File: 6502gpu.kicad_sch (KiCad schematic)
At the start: 1 part, among them J1 DE15_Receptacle_HighDensity

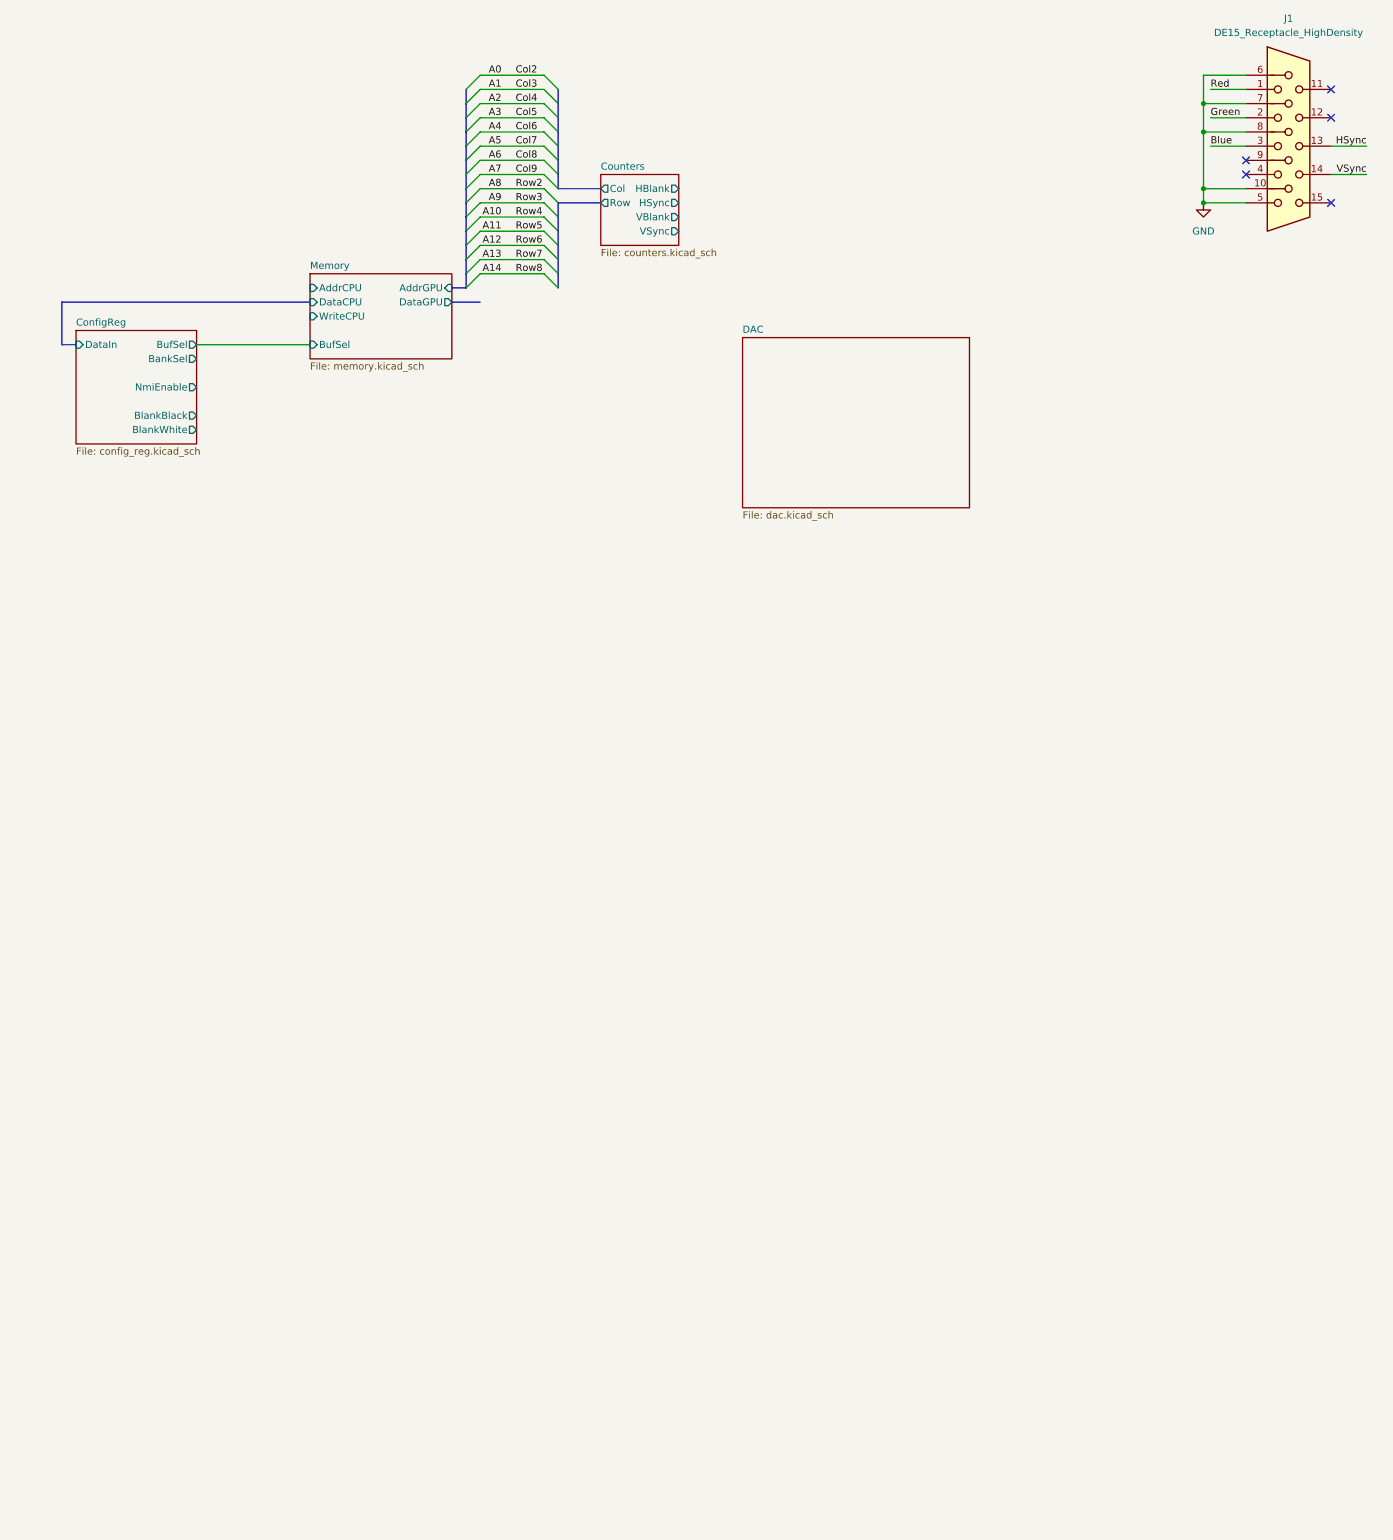
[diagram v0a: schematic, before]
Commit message: cleanup
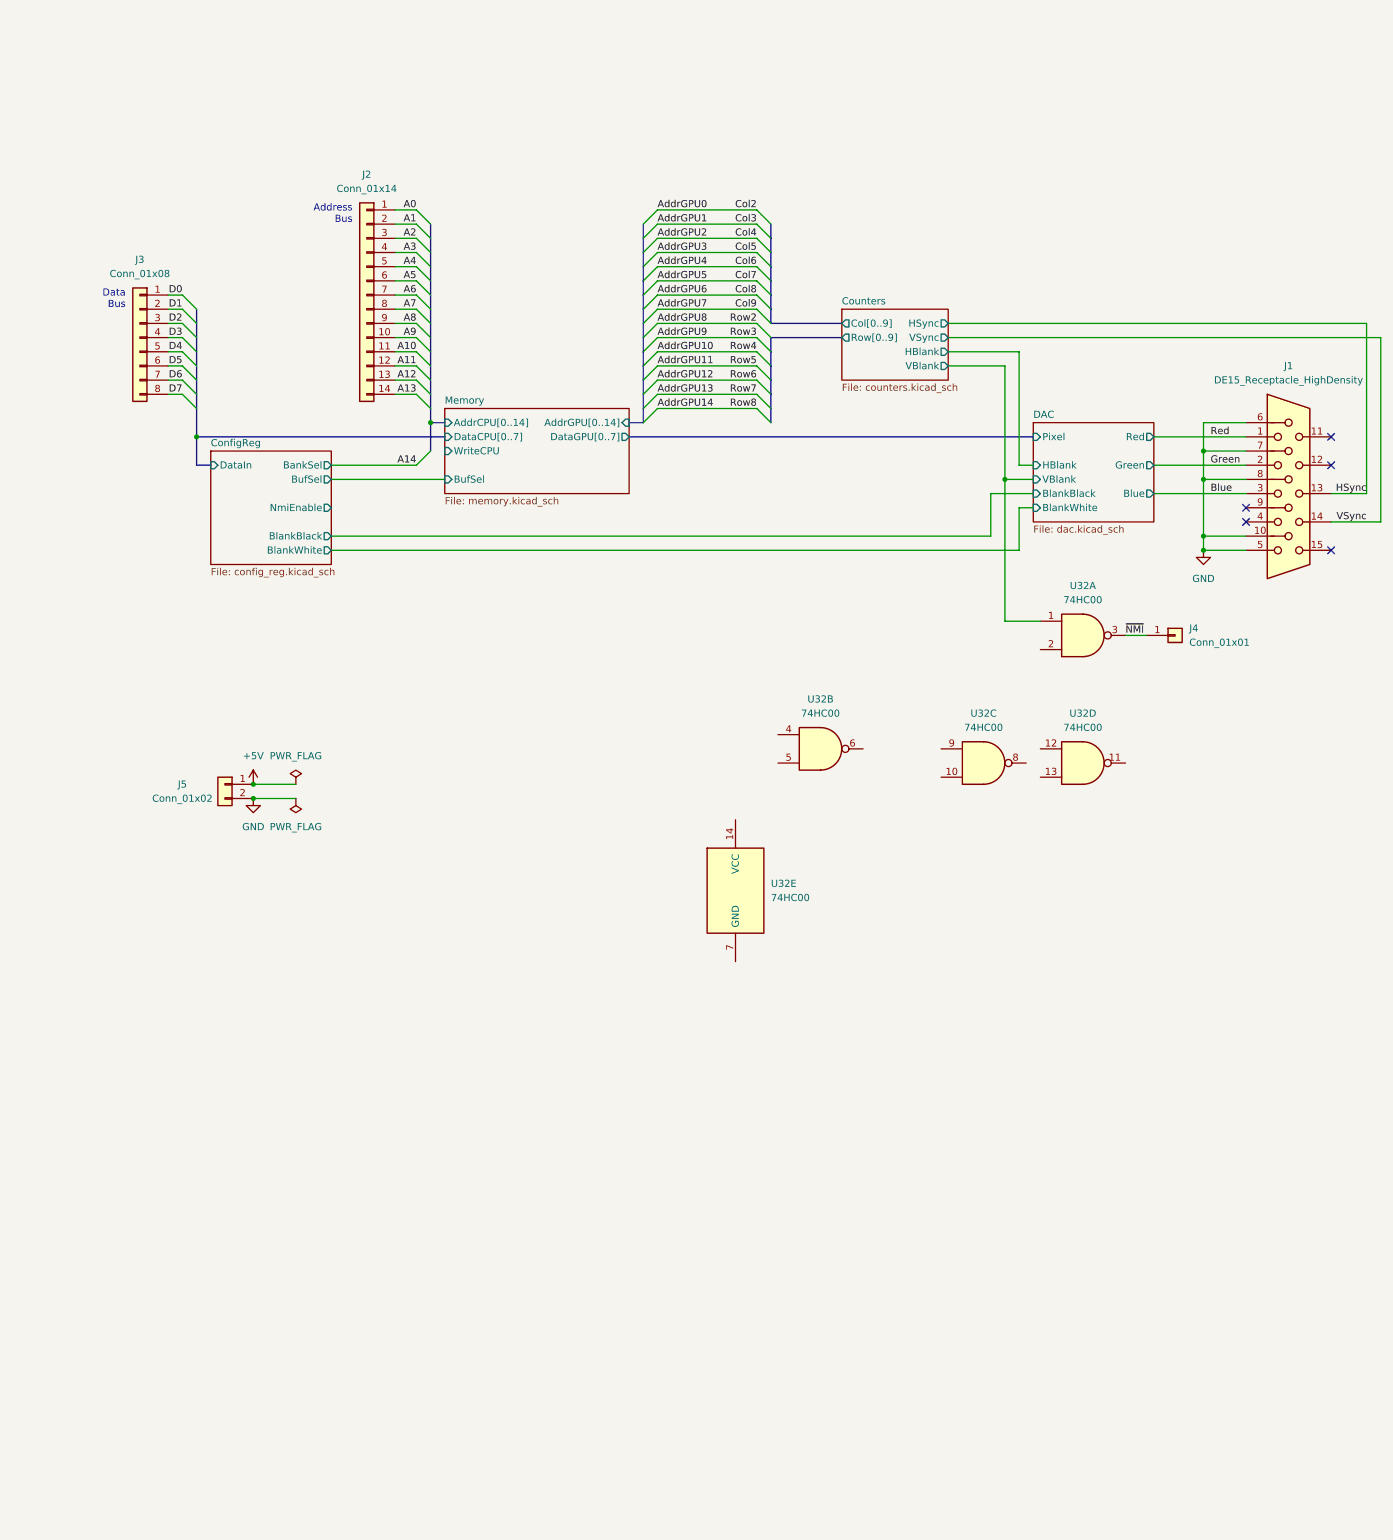
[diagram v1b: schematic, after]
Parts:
- added J2: Conn_01x14, symbol Connector_Generic:Conn_01x14
- added J3: Conn_01x08, symbol Connector_Generic:Conn_01x08
- added J4: Conn_01x01, symbol Connector_Generic:Conn_01x01
- added J5: Conn_01x02, symbol Connector_Generic:Conn_01x02
- added U32: 74HC00, symbol 74xx:74HC00
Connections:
- net A0: now also J2.1 (Pin_1)
- net A1: now also J2.2 (Pin_2)
- net A10: now also J2.11 (Pin_11)
- net A11: now also J2.12 (Pin_12)
- net A12: now also J2.13 (Pin_13)
- net A13: now also J2.14 (Pin_14)
- net A2: now also J2.3 (Pin_3)
- net A3: now also J2.4 (Pin_4)
- net A4: now also J2.5 (Pin_5)
- net A5: now also J2.6 (Pin_6)
- net A6: now also J2.7 (Pin_7)
- net A7: now also J2.8 (Pin_8)
- net A8: now also J2.9 (Pin_9)
- net A9: now also J2.10 (Pin_10)
- net Counters/VBlank: now also U32.1
- net GND: now also J5.2 (Pin_2)
- new net +5V: J5.1 (Pin_1)
- new net D0: J3.1 (Pin_1)
- new net D1: J3.2 (Pin_2)
- new net D2: J3.3 (Pin_3)
- new net D3: J3.4 (Pin_4)
- new net D4: J3.5 (Pin_5)
- new net D5: J3.6 (Pin_6)
- new net D6: J3.7 (Pin_7)
- new net D7: J3.8 (Pin_8)
- new net ~{NMI}: J4.1 (Pin_1), U32.3
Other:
- sheet Counters ports: added Col[0..9], Row[0..9]; removed Col, Row
- sheet DAC ports: added BlankBlack, BlankWhite, Blue, Green, HBlank, Pixel, Red, VBlank; removed none
- sheet Memory ports: added AddrCPU[0..14], AddrGPU[0..14], DataCPU[0..7], DataGPU[0..7]; removed AddrCPU, AddrGPU, DataCPU, DataGPU
- note added: "Address Bus"
- note added: "Data Bus"
- moved on the sheet: J1

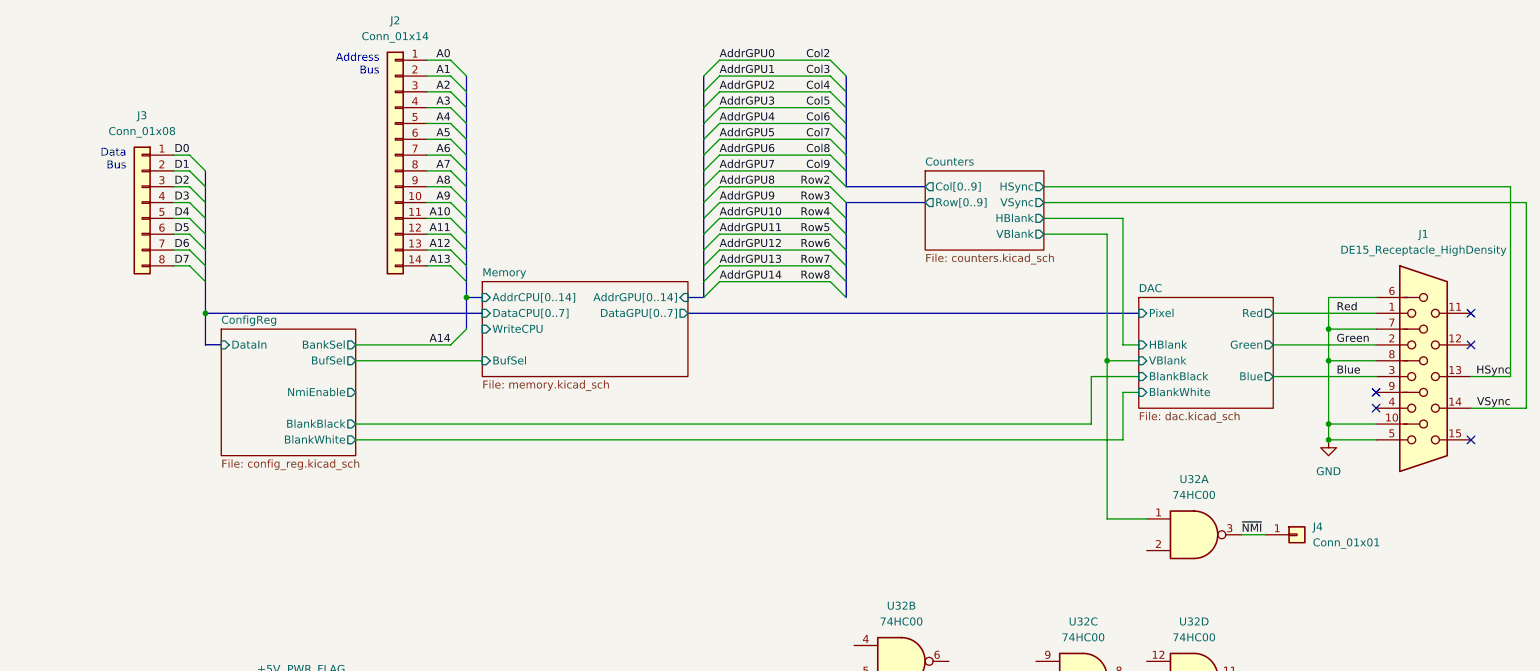
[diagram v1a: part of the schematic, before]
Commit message: remove 3390, cleanup
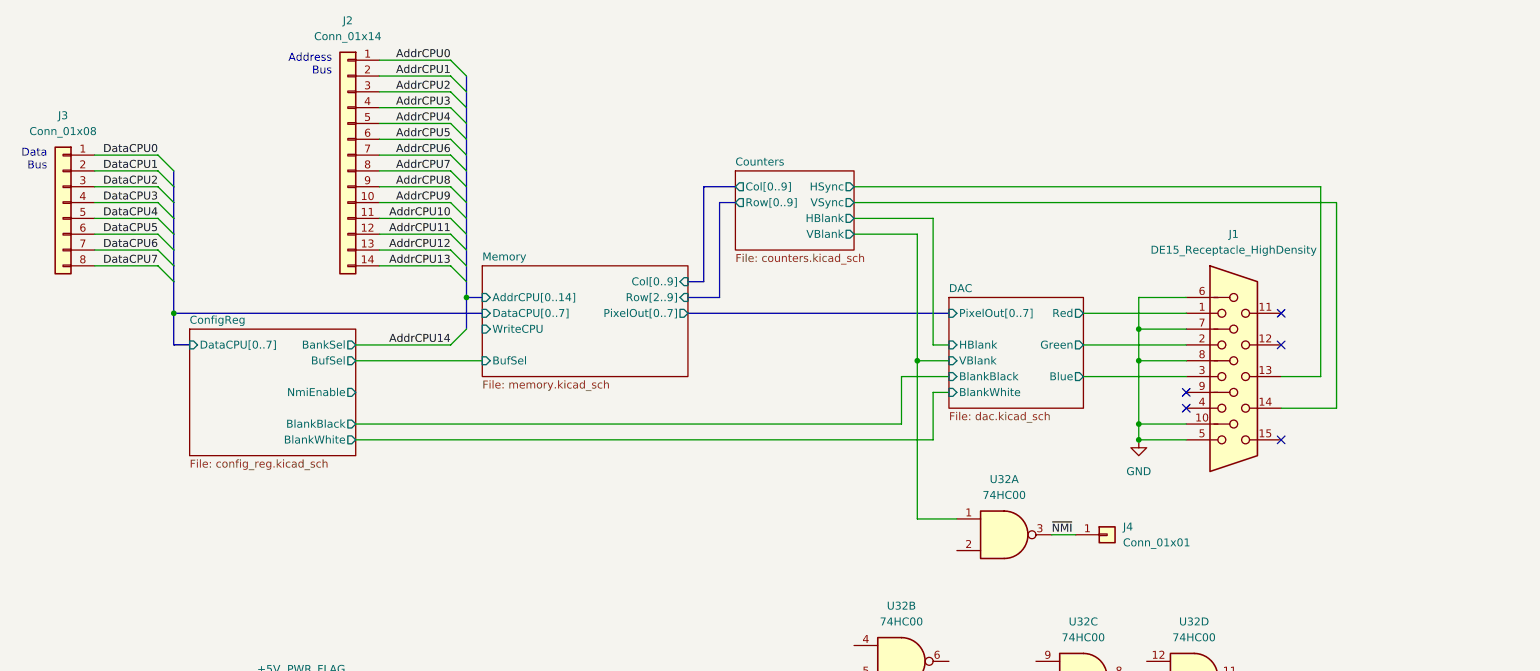
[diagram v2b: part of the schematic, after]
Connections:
- net A0 renamed AddrCPU0
- net A1 renamed AddrCPU1
- net A10 renamed AddrCPU10
- net A11 renamed AddrCPU11
- net A12 renamed AddrCPU12
- net A13 renamed AddrCPU13
- net A2 renamed AddrCPU2
- net A3 renamed AddrCPU3
- net A4 renamed AddrCPU4
- net A5 renamed AddrCPU5
- net A6 renamed AddrCPU6
- net A7 renamed AddrCPU7
- net A8 renamed AddrCPU8
- net A9 renamed AddrCPU9
- net Blue renamed DAC/Blue
- net D0 renamed DataCPU0
- net D1 renamed DataCPU1
- net D2 renamed DataCPU2
- net D3 renamed DataCPU3
- net D4 renamed DataCPU4
- net D5 renamed DataCPU5
- net D6 renamed DataCPU6
- net D7 renamed DataCPU7
- net Green renamed DAC/Green
- net HSync renamed Counters/HSync
- net Red renamed DAC/Red
- net VSync renamed Counters/VSync
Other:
- sheet ConfigReg ports: added DataCPU[0..7]; removed DataIn
- sheet DAC ports: added PixelOut[0..7]; removed Pixel
- sheet Memory ports: added Col[0..9], PixelOut[0..7], Row[2..9]; removed AddrGPU[0..14], DataGPU[0..7]
- moved on the sheet: J1, J2, J3, J4, U32A
